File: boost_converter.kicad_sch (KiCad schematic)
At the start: 15 parts, among them U4 TPS61088RHLR, U5 MCP4561-104E/MS

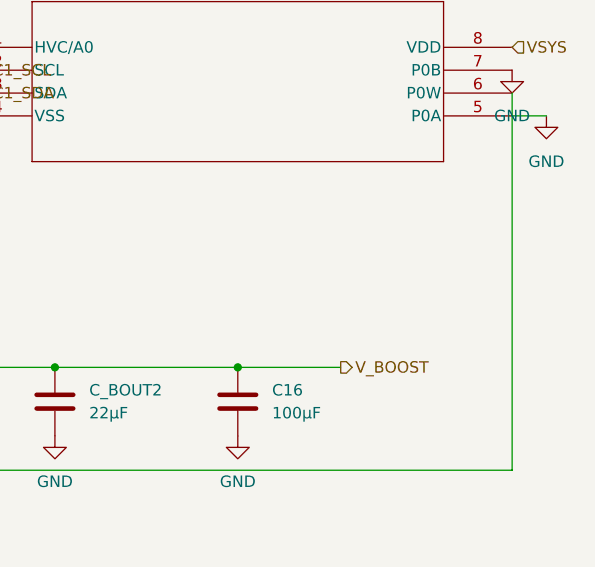
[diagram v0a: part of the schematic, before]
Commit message: finished schematics
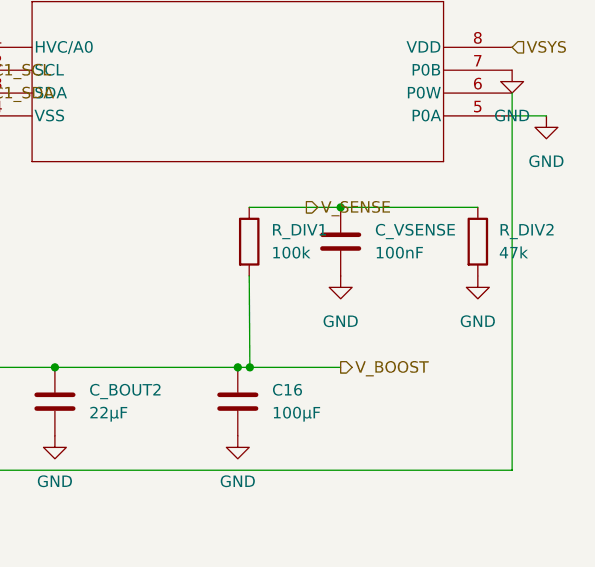
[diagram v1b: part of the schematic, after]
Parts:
- added C_VSENSE: 100nF, symbol Device:C
- added R_DIV1: 100k, symbol Device:R
- added R_DIV2: 47k, symbol Device:R
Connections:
- net GND: now also C_VSENSE.2, R_DIV2.2
- net V_BOOST: now also R_DIV1.2
- new net V_SENSE: C_VSENSE.1, R_DIV1.1, R_DIV2.1
